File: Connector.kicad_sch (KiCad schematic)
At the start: 1 part, among them J3 TC2070-IDC-NL

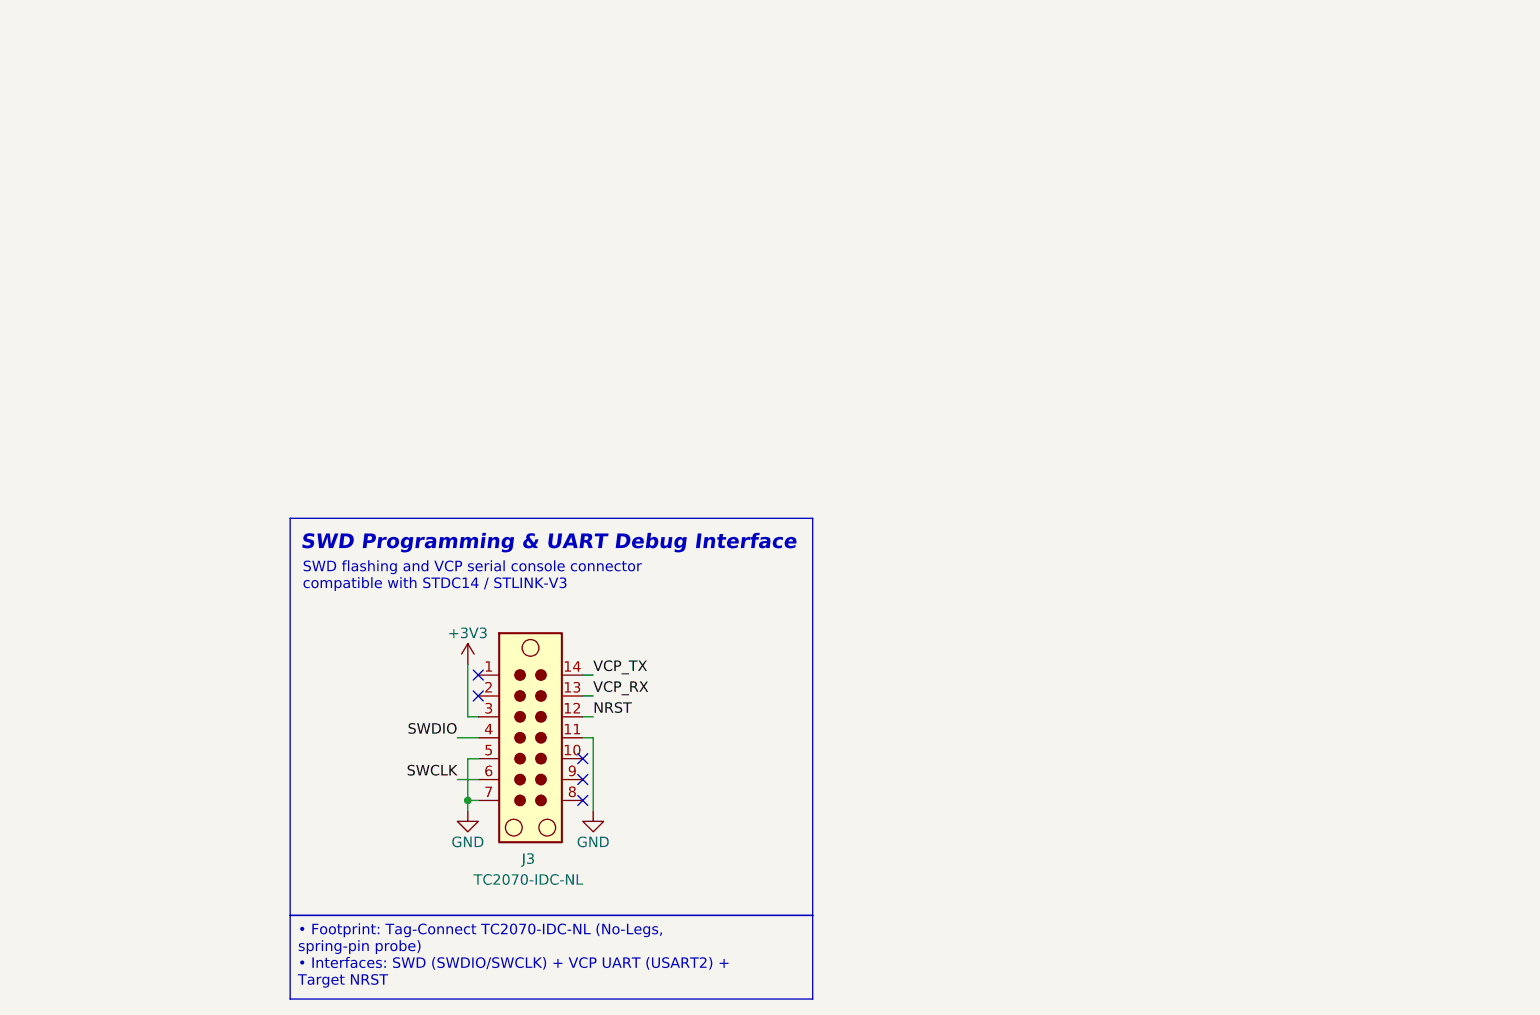
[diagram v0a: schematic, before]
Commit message: fix: fix some errors in shematic
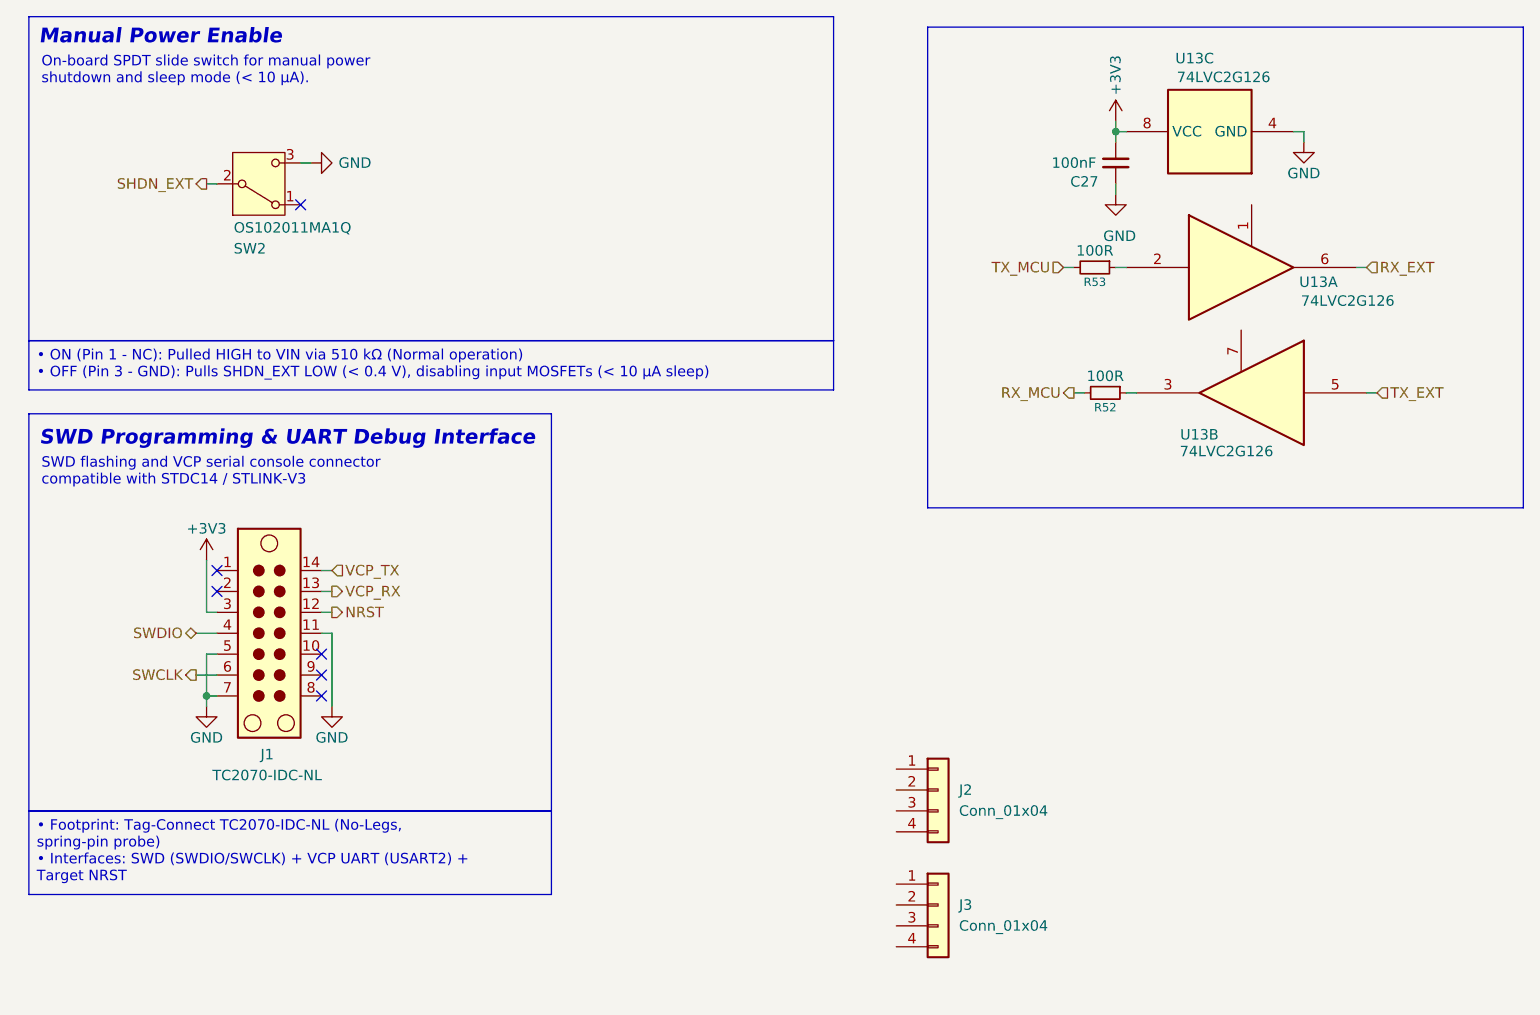
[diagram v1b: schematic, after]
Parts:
- added C27: 100nF, Capacitor_SMD:C_0603_1608Metric, symbol Device:C_Small
- added J2: Conn_01x04, Connector_Wire:SolderWire-1sqmm_1x04_P7.8mm_D1.4mm_OD3.9mm_Relief, symbol Connector_Generic:Conn_01x04
- added J3: Conn_01x04, Connector_JST:JST_XH_S4B-XH-A-1_1x04_P2.50mm_Horizontal, symbol Connector_Generic:Conn_01x04
- added R52, R53: 100R, Resistor_SMD:R_0603_1608Metric, symbol Device:R_Small
- added SW2: OS102011MA1Q, Button_Switch_THT:SW_Slide_SPDT_Angled_CK_OS102011MA1Q, symbol Switch:SW_SPDT
- added U13: 74LVC2G126, Package_SO:VSSOP-8_2.3x2mm_P0.5mm, symbol 74xGxx:74LVC2G126
- J1: renamed from J3; footprint Library:Tag-Connect_TC2070-IDC-FP_2x07_P1.27mm_Vertical -> KineticCore:Tag-Connect_TC2070-IDC-FP_2x07_P1.27mm_Vertical
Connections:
- net +3V3: now also C27.1, U13.8 (VCC)
- net GND: now also C27.2, SW2.3 (C), U13.4 (GND)
- new net: R53.1, U13.2
- new net: R52.1, U13.3
- new net RX_EXT: U13.6
- new net RX_MCU: R52.2
- new net SHDN_EXT: SW2.2 (B)
- new net TX_EXT: U13.5
- new net TX_MCU: R53.2
- no-connect marks 5 -> 6
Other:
- note added: "Manual Power Enable"
- note added: "On-board SPDT slide switch for manual power shutdown and sleep mode (< 10 µA)."
- moved on the sheet: J1
